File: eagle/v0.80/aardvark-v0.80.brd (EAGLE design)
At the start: 100 x 98.9 mm, 34 parts, among them IC1 LM1117-3.3, J1 USB_MINI-B_SMT, U1 CH340C

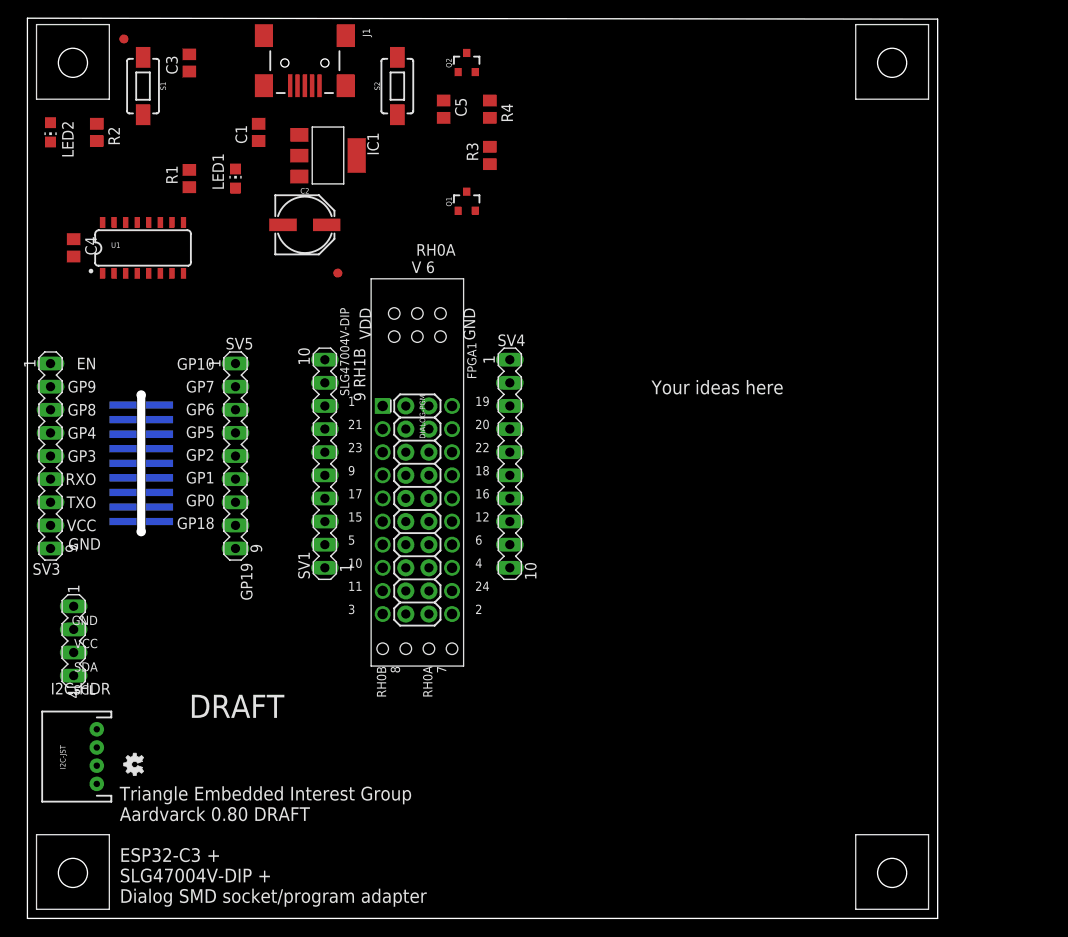
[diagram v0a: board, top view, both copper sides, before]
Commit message: example usage of v0.80 shown with aardvark-v0.80-board.pdf
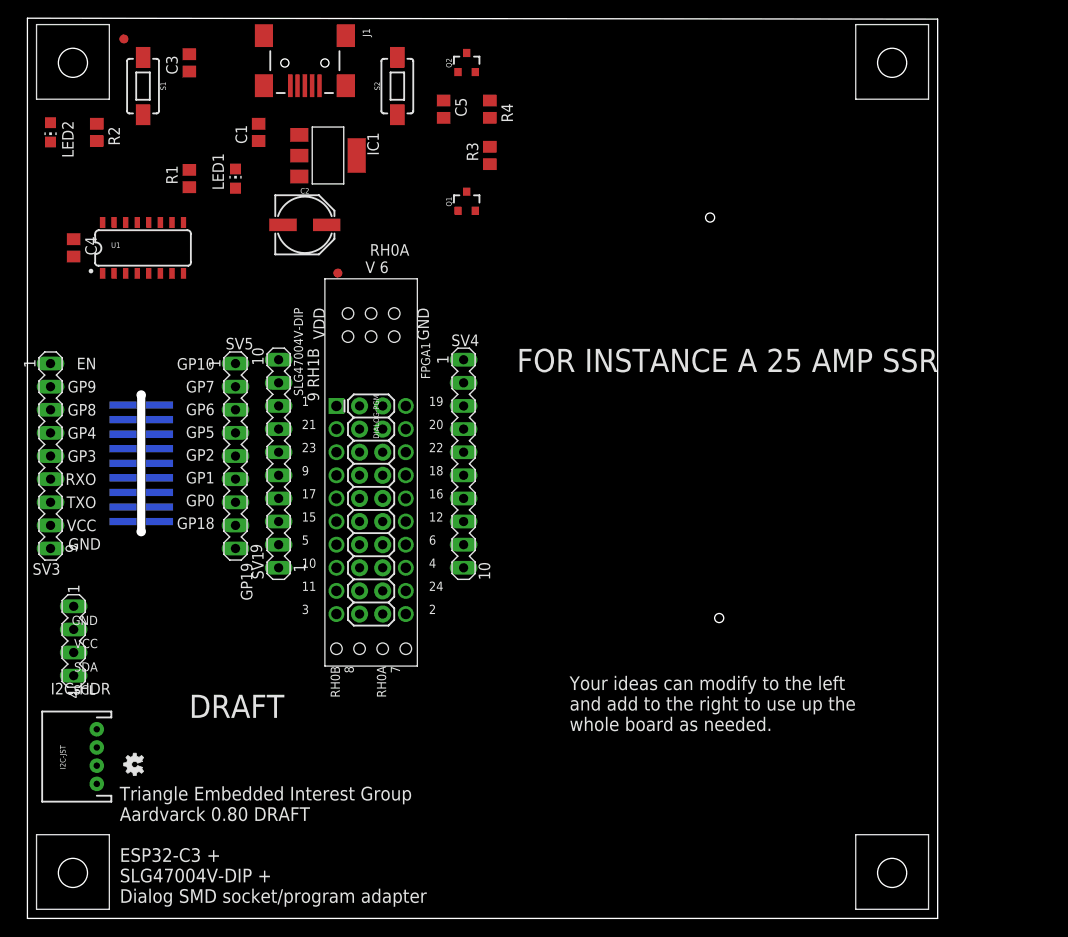
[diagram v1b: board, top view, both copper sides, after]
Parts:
- moved FPGA1 5.08 mm to (37.8, 51.2)
- moved DIALOG-PGM 5.08 mm to (36.5, 56.3)
- moved SV1 5.08 mm to (27.6, 50.0)
- moved SV4 5.08 mm to (47.9, 50.0)
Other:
- board text added: "FOR INSTANCE A 25 AMP SSR"
- board text added: "Your ideas can modify to the left and add to the right to use up the whole board as needed."
- board text removed: "Your ideas here"
